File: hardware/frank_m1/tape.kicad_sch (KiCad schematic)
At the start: 11 parts, among them J11 SJ1-353XNG, Q1 BC850, Q2 BC850

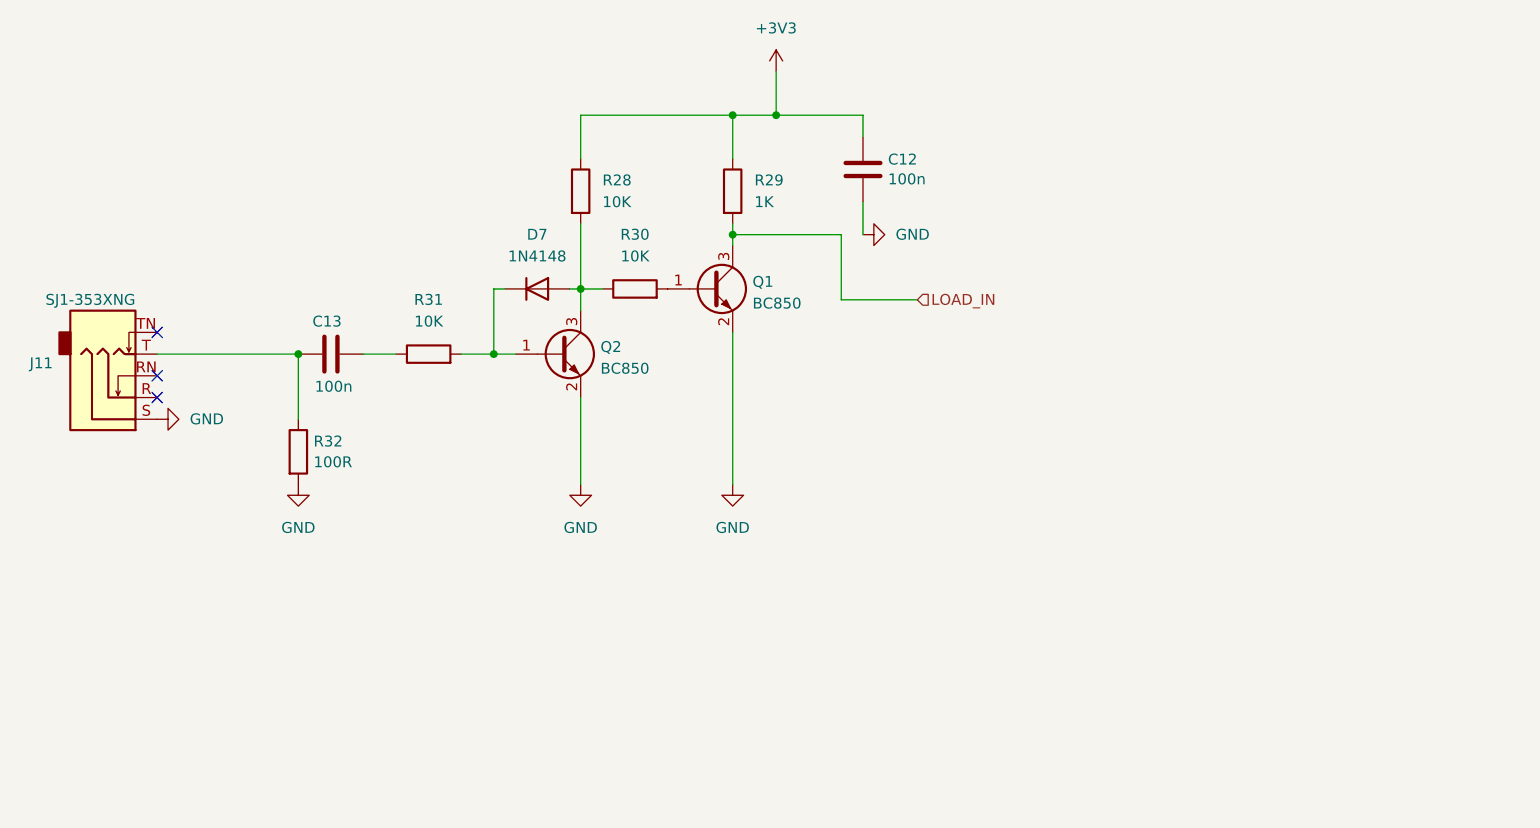
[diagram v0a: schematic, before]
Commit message: Minor updates
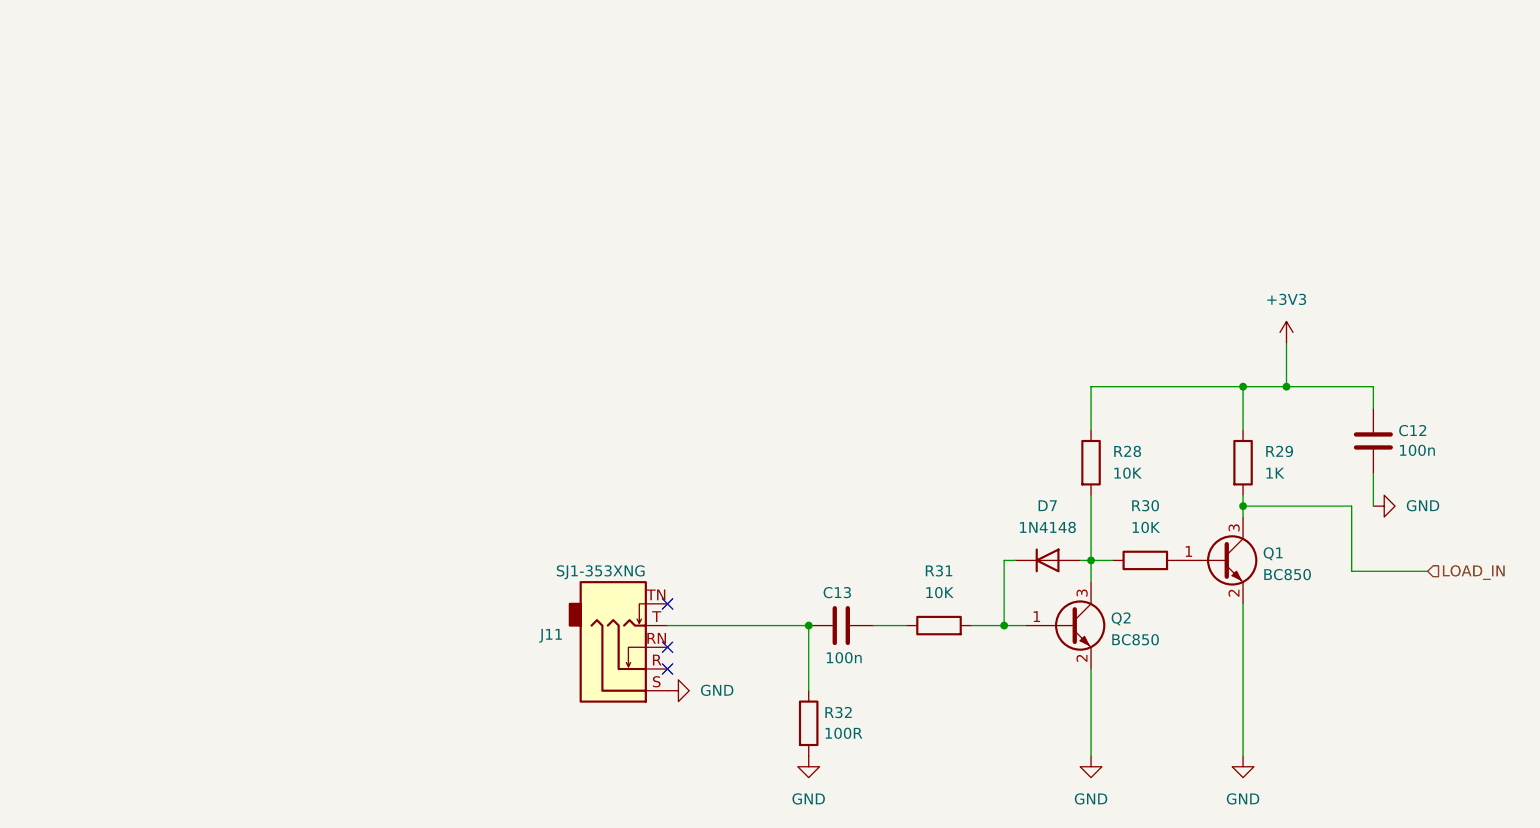
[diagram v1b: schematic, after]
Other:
- moved on the sheet: C12, C13, D7, J11, Q1, Q2, R28, R29, R30, R31, R32
